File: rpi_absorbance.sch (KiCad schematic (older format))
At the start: 35 parts, among them P1 CONN_01X02, P2 CONN_01X06, P3 RPI_HEADER, P4 CONN_01X04, P5 CONN_01X03, Q1 NPN, U1 R-78B5.0-1.5L, U2 MEE1S1212SC, U3 DRV8825, U4 TCA9406DCUR

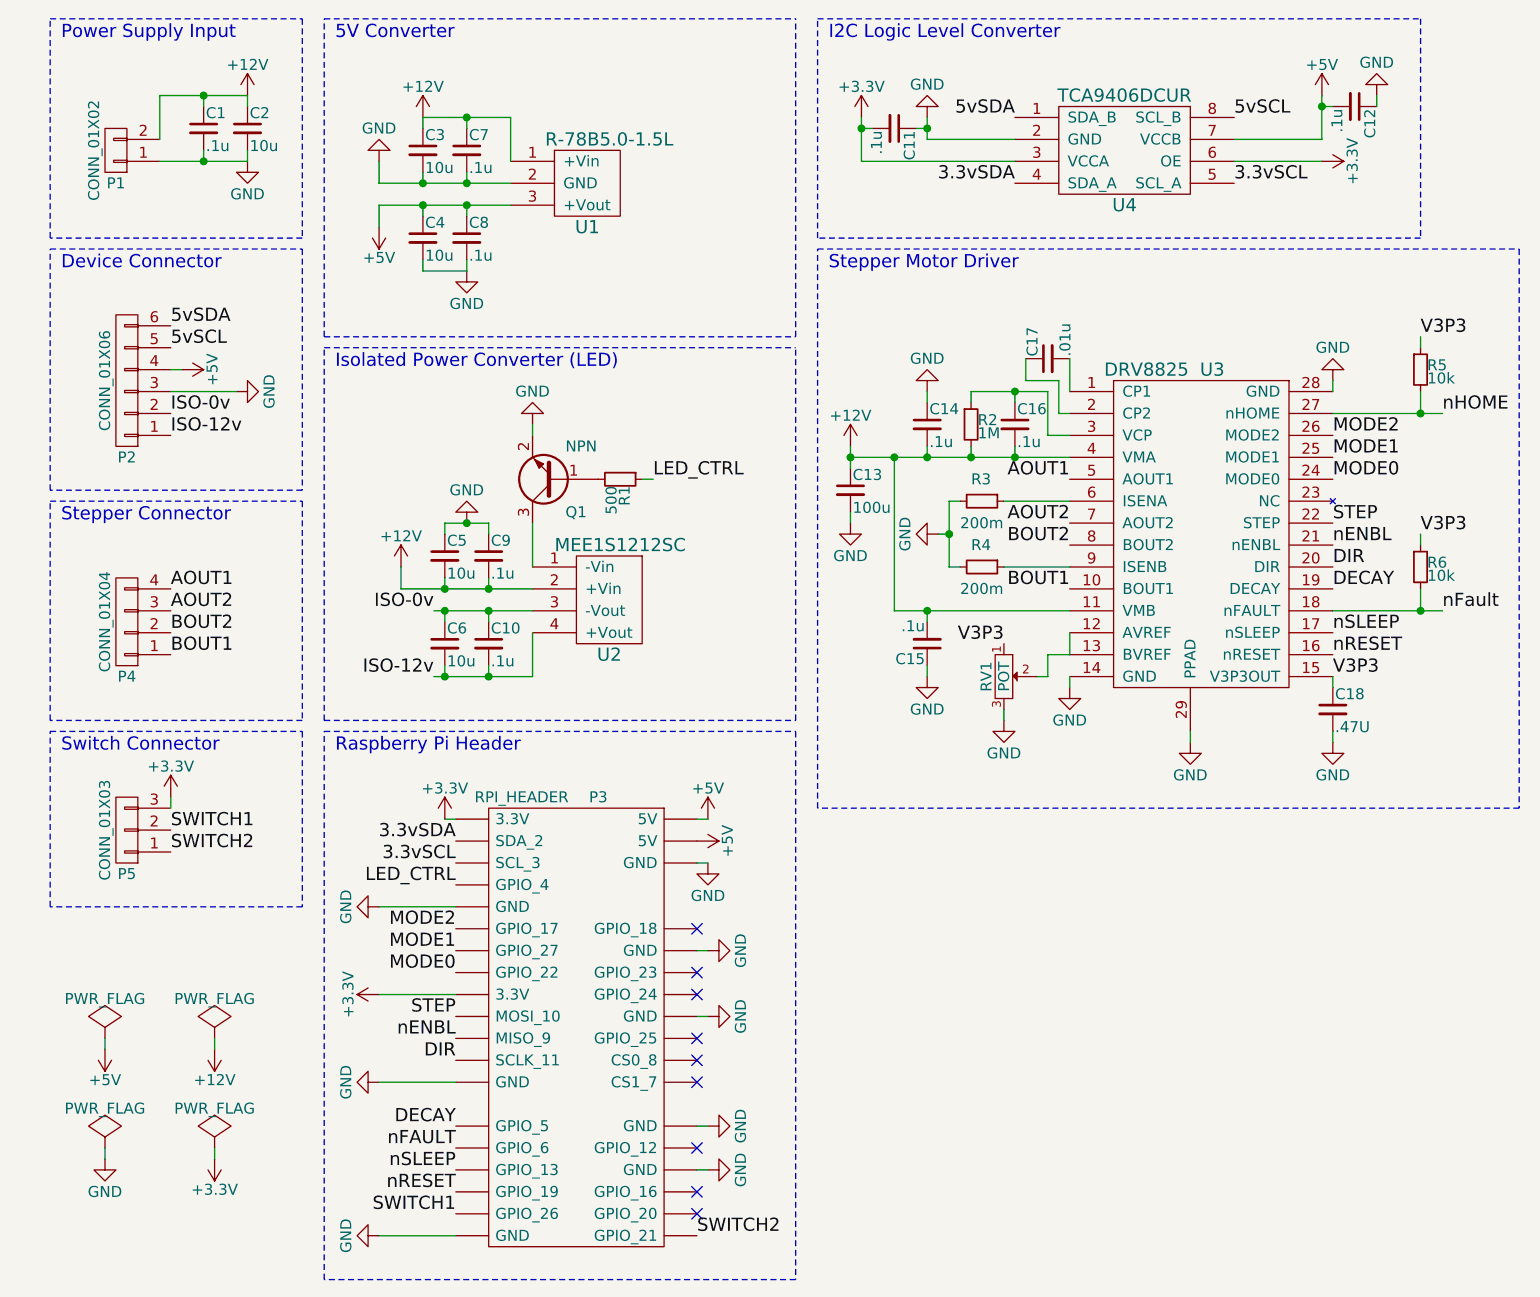
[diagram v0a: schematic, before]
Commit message: Add components
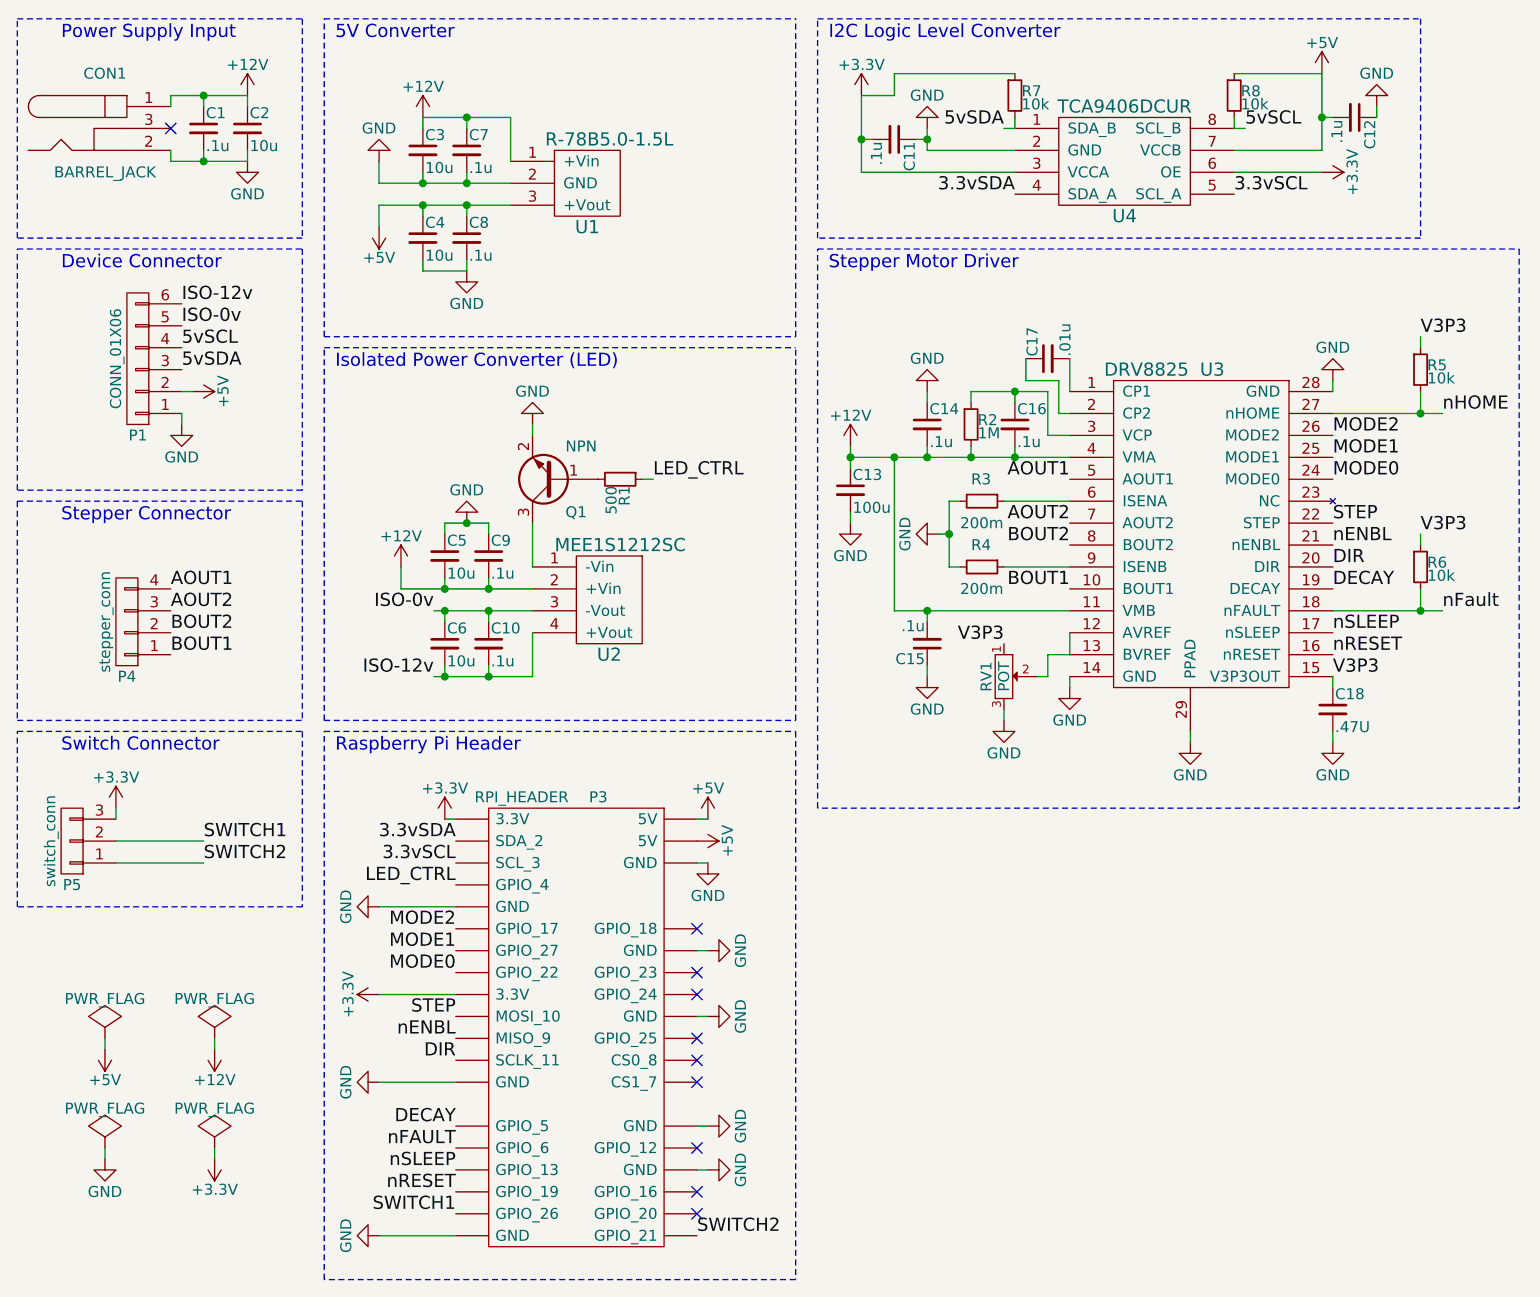
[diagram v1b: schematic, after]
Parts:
- removed P1: CONN_01X02, symbol CONN_01X02
- removed P2: CONN_01X06, symbol CONN_01X06
- added CON1: BARREL_JACK, footprints:CUI_BARREL_JACK, symbol BARREL_JACK
- added P1: CONN_01X06, Pin_Headers:Pin_Header_Straight_1x06, symbol CONN_01X06
- added R7, R8: 10k, Resistors_SMD:R_0805_HandSoldering, symbol R_Small
- C1, C10, C11, C12, C14, C15, C16, C17, C18, C2, C3, C4, C5, C6, C7, C8, C9: footprint (none) -> Capacitors_SMD:C_0603
- C13: footprint (none) -> Capacitors_SMD:c_elec_8x6.7
- P3: footprint (none) -> Pin_Headers:Pin_Header_Straight_2x20
- P4: value CONN_01X04 -> stepper_conn; footprint (none) -> Pin_Headers:Pin_Header_Straight_1x04
- P5: value CONN_01X03 -> switch_conn; footprint (none) -> Pin_Headers:Pin_Header_Straight_1x03
- Q1: footprint (none) -> TO_SOT_Packages_SMD:SOT-23
- R1, R2, R3, R4, R5, R6: footprint (none) -> Resistors_SMD:R_0603
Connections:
- net +12V: now also CON1.1
- net +3V3: now also R7.1
- net +5V: now also P1.2 (P2), R8.1
- net 5vSCL: now also P1.4 (P4), R8.2
- net 5vSDA: now also P1.3 (P3), R7.2
- net GND: now also CON1.2, P1.1 (P1)
- net ISO-0v: now also P1.5 (P5)
- net ISO-12v: now also P1.6 (P6)
- no-connect marks 9 -> 10
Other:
- moved on the sheet: C11, C12, P5, U4
